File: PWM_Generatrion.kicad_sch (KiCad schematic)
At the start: 3 parts, among them J13 DF11-10DP-2DSA24, J14 DF11-10DP-2DSA24, U22 PCA9685PW_118

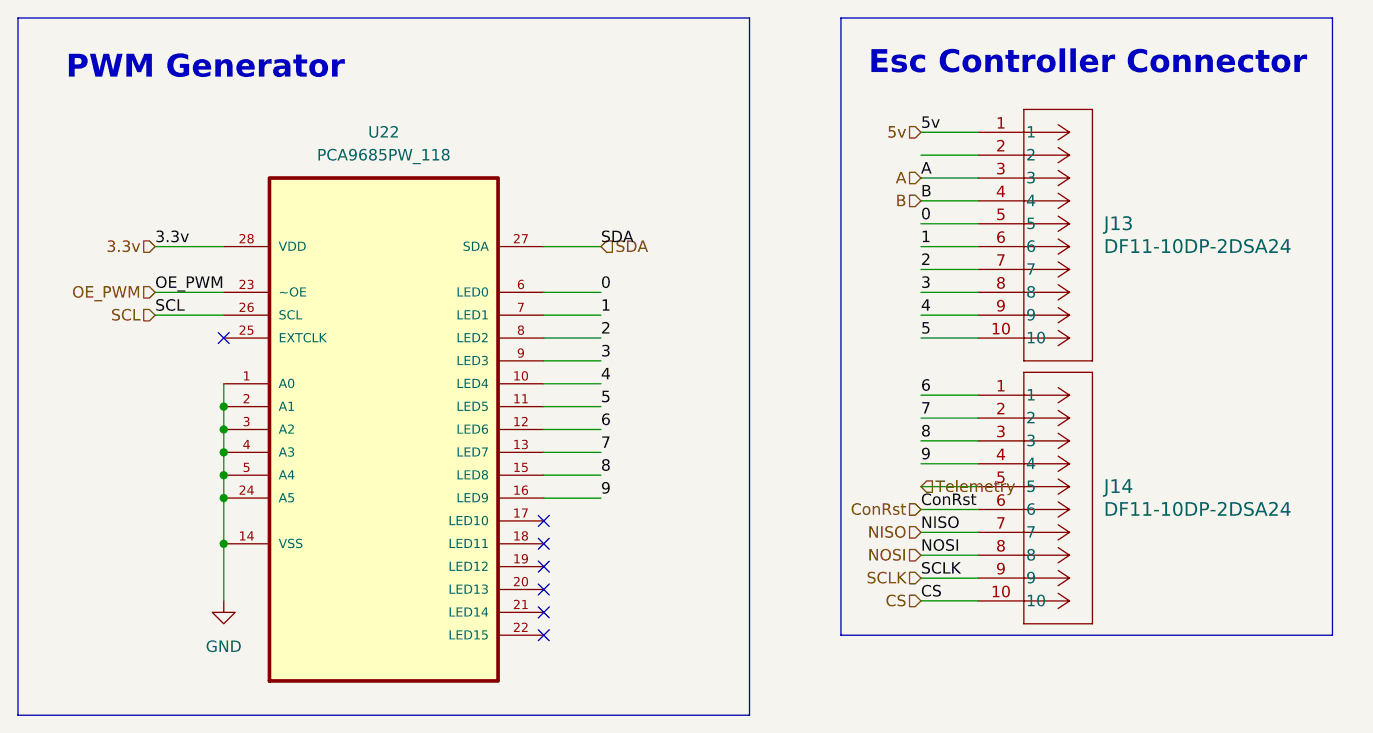
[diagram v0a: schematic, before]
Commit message: stuff
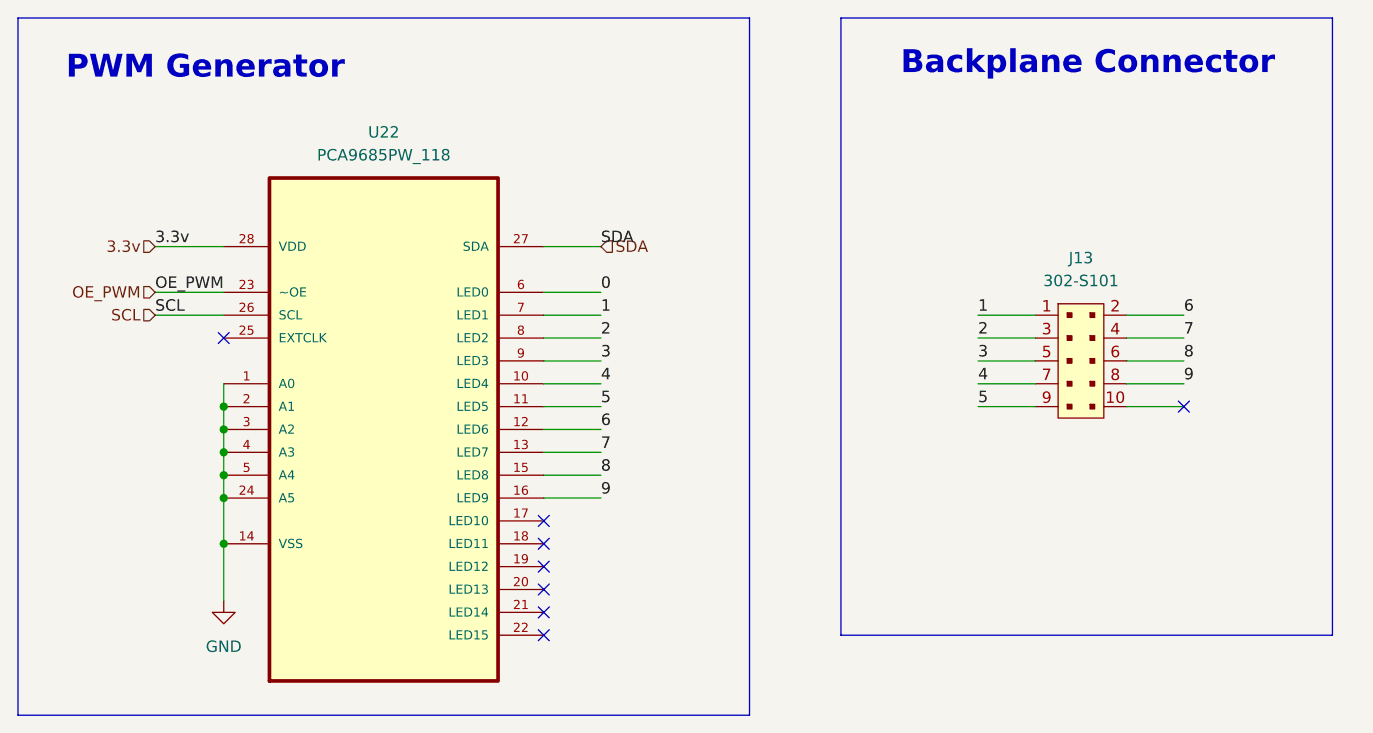
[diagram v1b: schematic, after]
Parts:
- removed J13, J14: DF11-10DP-2DSA24, CON10_2X5_UF_DF11_HIR, symbol DF11_10DP_2DSA:DF11-10DP-2DSA24
- added J13: 302-S101, digikey-footprints:PinHeader_2x5_P2.54mm_Drill1.2mm, symbol dk_Rectangular-Connectors-Headers-Male-Pins:302-S101
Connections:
- net 1: now also J13.1
- net 2: now also J13.3
- net 3: now also J13.5
- net 4: now also J13.7
- net 5: now also J13.9
- net 6: now also J13.2
- net 7: now also J13.4
- net 8: now also J13.6
- net 9: now also J13.8
- no-connect marks 7 -> 8
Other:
- note added: "Backplane Connector"
- note removed: "Esc Controller Connector"
